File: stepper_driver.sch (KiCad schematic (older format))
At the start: 83 parts, among them IC1 TMC2160-TA, J1 BARREL_JACK, J2 Screw_Terminal_01x04, J3 CONN_02X07, J4 CONN_01X04, J9 USB_C_Receptacle_USB2.0, Q1 Q_NPN_BEC, Q2 Si4946BEY, Q3 Si4946BEY, Q4 Q_NPN_BEC, Q5 Si4946BEY, Q6 Si4946BEY, SW1 SW_Push, SW2 SW_Push, U1 CH340B, U2 XC6210B332MR, U3 XL1509-5.0, U4 ESP32-WROOM-32D, U6 SN74LV1T34DBV

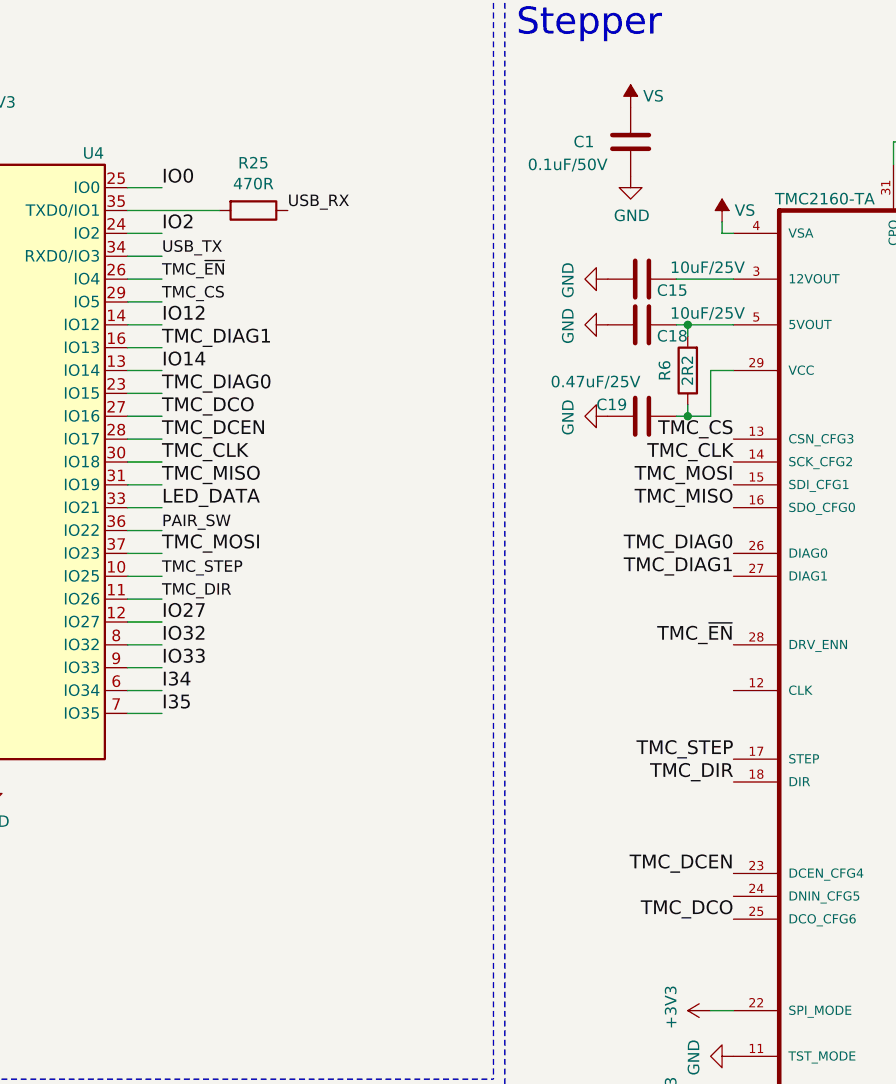
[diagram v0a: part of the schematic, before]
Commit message: Minor board updates
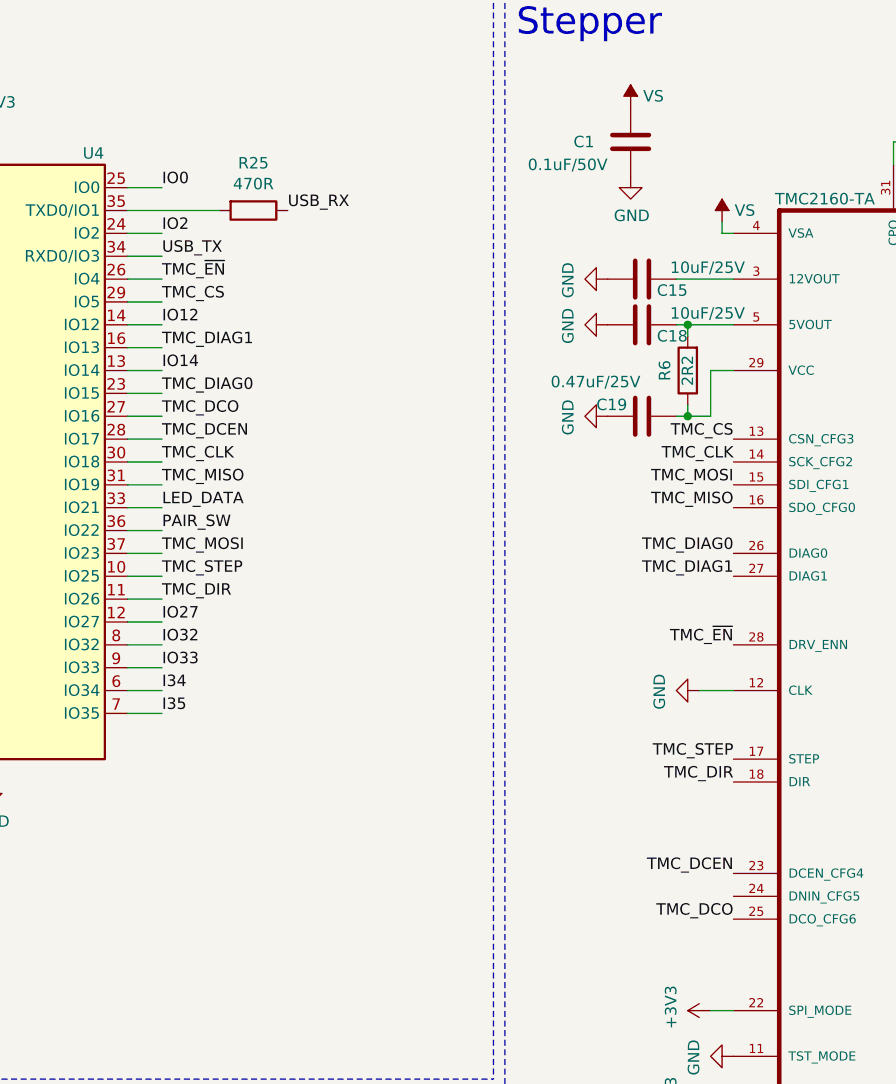
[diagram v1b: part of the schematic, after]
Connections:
- net GND: now also IC1.12 (CLK)
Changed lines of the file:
@@
 Text Label 7250 1900 0    50   ~ 0
 USB_RX
-Text Label 6700 2100 0    50   ~ 0
-USB_TX
 $Comp
 L Switch:SW_Push SW?
@@
 Wire Notes Line
 	4150 950  8150 950
-Text Label 6700 3200 0    60   ~ 0
+Text Label 6700 3200 0    50   ~ 0
 LED_DATA
-Text Label 6700 3400 0    60   ~ 0
+Text Label 6700 3400 0    50   ~ 0
 TMC_MOSI
 $Comp
@@
 Wire Wire Line
 	5200 1800 5350 1800
-Text Label 6700 1800 0    60   ~ 0
+Text Label 6700 1800 0    50   ~ 0
 IO0
 Wire Wire Line
@@
 Wire Wire Line
 	6550 1900 6950 1900
-Text Label 6700 2300 0    50   ~ 0
-TMC_CS
 Wire Wire Line
 	6550 4100 6700 4100
@@
 	1    0    0    -1
 $EndComp
-Text Label 9200 3800 2    60   ~ 0
+Text Label 9200 3800 2    50   ~ 0
 TMC_~EN
 $Comp
@@
 	1    0    0    -1
 $EndComp
-Text Label 6700 3100 0    60   ~ 0
-TMC_MISO
-Text Label 6700 3000 0    60   ~ 0
+Text Label 9200 2900 2    50   ~ 0
+TMC_CS
+Text Label 9200 3000 2    50   ~ 0
 TMC_CLK
-Text Label 9200 2900 2    60   ~ 0
-TMC_CS
-Text Label 6700 2200 0    50   ~ 0
-TMC_~EN
-Text Label 9200 3000 2    60   ~ 0
-TMC_CLK
-Text Label 9200 3100 2    60   ~ 0
+Text Label 9200 3100 2    50   ~ 0
 TMC_MOSI
-Text Label 9200 3200 2    60   ~ 0
+Text Label 9200 3200 2    50   ~ 0
 TMC_MISO
 Text Label 12550 4000 2    50   ~ 0
@@
 Text Label 14850 5800 2    50   ~ 0
 BMA2
-Text Label 6700 3700 0    60   ~ 0
+Text Label 6700 3700 0    50   ~ 0
 IO27
-Text Label 9200 4400 2    60   ~ 0
+Text Label 9200 4400 2    50   ~ 0
 TMC_DIR
 Text Label 6700 3600 0    50   ~ 0
 TMC_DIR
-Text Label 9200 4300 2    60   ~ 0
+Text Label 9200 4300 2    50   ~ 0
 TMC_STEP
 Text Label 6700 3500 0    50   ~ 0
@@
 Text Label 5250 2100 2    50   ~ 0
 I39
-Text Label 6700 4000 0    60   ~ 0
+Text Label 6700 4000 0    50   ~ 0
 I34
-Text Label 6700 4100 0    60   ~ 0
+Text Label 6700 4100 0    50   ~ 0
 I35
-Text Label 6700 3800 0    60   ~ 0
+Text Label 6700 3800 0    50   ~ 0
 IO32
-Text Label 6700 3900 0    60   ~ 0
+Text Label 6700 3900 0    50   ~ 0
 IO33
 Wire Wire Line
@@
 Wire Wire Line
 	6700 2900 6550 2900
-Text Label 6700 2000 0    60   ~ 0
-IO2
 Wire Wire Line
 	6550 1800 6700 1800
@@
 Text Label 5250 2000 2    50   ~ 0
 VS_SENSE
-Text Label 6700 2400 0    60   ~ 0
-IO12
 Wire Wire Line
 	6700 2400 6550 2400
-Text Label 6700 2600 0    60   ~ 0
-IO14
 Wire Wire Line
 	6700 2600 6550 2600
@@
 	1    0    0    -1
 $EndComp
-Text Label 9200 4800 2    60   ~ 0
+Text Label 9200 4800 2    50   ~ 0
 TMC_DCEN
-Text Label 9200 5000 2    60   ~ 0
+Text Label 9200 5000 2    50   ~ 0
 TMC_DCO
-Text Label 6700 2900 0    60   ~ 0
+Text Label 9200 3400 2    50   ~ 0
+TMC_DIAG0
+Text Label 9200 3500 2    50   ~ 0
+TMC_DIAG1
+Wire Notes Line
+	8200 6750 15850 6750
+Wire Notes Line
+	15850 6750 15850 950
+Wire Notes Line
+	8200 950  8200 6750
+Wire Notes Line
+	8200 950  15850 950
+Wire Notes Line
+	11550 8850 11550 9900
+Wire Notes Line
+	9700 8850 11550 8850
+Wire Notes Line
+	9700 9900 11550 9900
+$Comp
+L power:GND #PWR0182
+U 1 1 6277F220
+P 9050 4000
+F 0 "#PWR0182" H 9050 3750 50  0001 C CNN
+F 1 "GND" H 9055 3827 50  0000 C CNN
+F 2 "" H 9050 4000 50  0001 C CNN
+F 3 "" H 9050 4000 50  0001 C CNN
+	1    9050 4000
+	0    1    1    0
+$EndComp
+Wire Wire Line
+	9050 4000 9200 4000
+Text Label 6700 2500 0    50   ~ 0
+TMC_DIAG1
+Text Label 6700 2700 0    50   ~ 0
+TMC_DIAG0
+Text Label 6700 2800 0    50   ~ 0
+TMC_DCO
+Text Label 6700 2900 0    50   ~ 0
 TMC_DCEN
-Text Label 6700 2800 0    60   ~ 0
-TMC_DCO
-Text Label 9200 3400 2    60   ~ 0
-TMC_DIAG0
-Text Label 9200 3500 2    60   ~ 0
-TMC_DIAG1
-Text Label 6700 2700 0    60   ~ 0
-TMC_DIAG0
-Text Label 6700 2500 0    60   ~ 0
-TMC_DIAG1
-Wire Notes Line
-	8200 6750 15850 6750
-Wire Notes Line
-	15850 6750 15850 950
-Wire Notes Line
-	8200 950  8200 6750
-Wire Notes Line
-	8200 950  15850 950
-Wire Notes Line
-	11550 8850 11550 9900
-Wire Notes Line
-	9700 8850 11550 8850
-Wire Notes Line
-	9700 9900 11550 9900
+Text Label 6700 2600 0    50   ~ 0
+IO14
+Text Label 6700 2400 0    50   ~ 0
+IO12
+Text Label 6700 2000 0    50   ~ 0
+IO2
+Text Label 6700 2200 0    50   ~ 0
+TMC_~EN
+Text Label 6700 3000 0    50   ~ 0
+TMC_CLK
+Text Label 6700 3100 0    50   ~ 0
+TMC_MISO
+Text Label 6700 2300 0    50   ~ 0
+TMC_CS
+Text Label 6700 2100 0    50   ~ 0
+USB_TX
 $EndSCHEMATC
